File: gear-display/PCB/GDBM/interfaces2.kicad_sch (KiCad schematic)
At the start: 4 parts, among them J6 Con_Screw_1x04_691313510004, J7 Con_Screw_1x04_691313510004

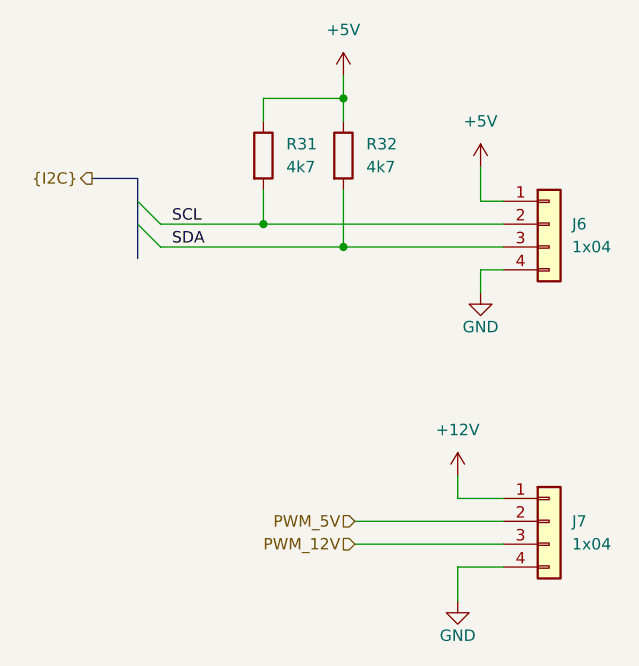
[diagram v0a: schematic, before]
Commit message: Layout
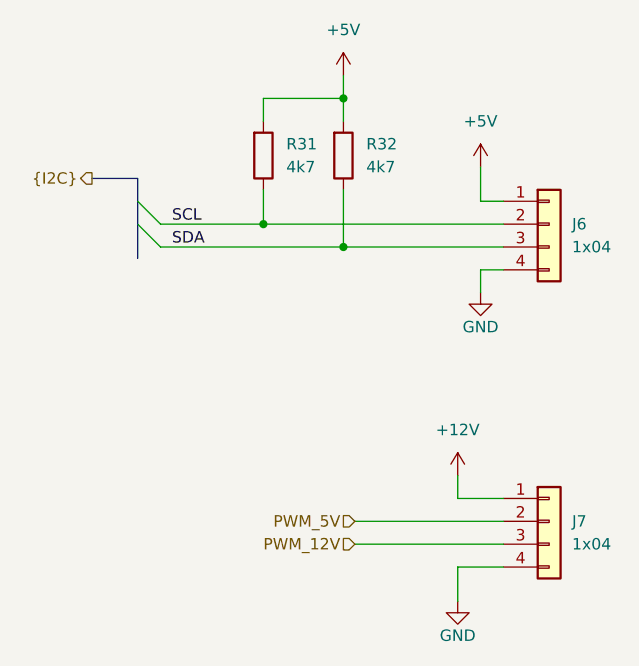
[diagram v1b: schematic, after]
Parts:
- J6, J7: value Con_Screw_1x04_691313510004 -> 1x04
- R31, R32: value R_0402_4700_1% -> 4k7
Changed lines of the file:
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@@
       (effects (font (size 1.27 1.27)) (justify left))
     )
-    (property "Value" "R_0402_4700_1%" (at 120.65 40.64 0)
+    (property "Value" "4k7" (at 120.65 40.64 0)
       (effects (font (size 1.27 1.27)) (justify left) hide)
     )
@@
       (effects (font (size 1.27 1.27)) (justify left))
     )
-    (property "Value" "Con_Screw_1x04_691313510004" (at 138.43 78.74 0)
+    (property "Value" "1x04" (at 138.43 78.74 0)
       (effects (font (size 1.27 1.27)) (justify left) hide)
     )
@@
       (effects (font (size 1.27 1.27)) (justify left))
     )
-    (property "Value" "Con_Screw_1x04_691313510004" (at 138.43 45.72 0)
+    (property "Value" "1x04" (at 138.43 45.72 0)
       (effects (font (size 1.27 1.27)) (justify left) hide)
     )
@@
       (effects (font (size 1.27 1.27)) (justify left))
     )
-    (property "Value" "R_0402_4700_1%" (at 111.76 40.64 0)
+    (property "Value" "4k7" (at 111.76 40.64 0)
       (effects (font (size 1.27 1.27)) (justify left) hide)
     )
